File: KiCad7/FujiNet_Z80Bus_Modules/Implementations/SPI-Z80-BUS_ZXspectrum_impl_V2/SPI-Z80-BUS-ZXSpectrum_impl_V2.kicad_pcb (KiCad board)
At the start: 2 copper layers, 155 x 55 mm, 28 parts, among them J1 PinHeader_2.54mm, J2 LOCAL_D, J3 ESP_SPI_INT, J4 ESP_CONTROL, J5 Z80_CONTROL, J6 LOCAL_A-L, J7 LOCAL_A-H, U1 74HC00

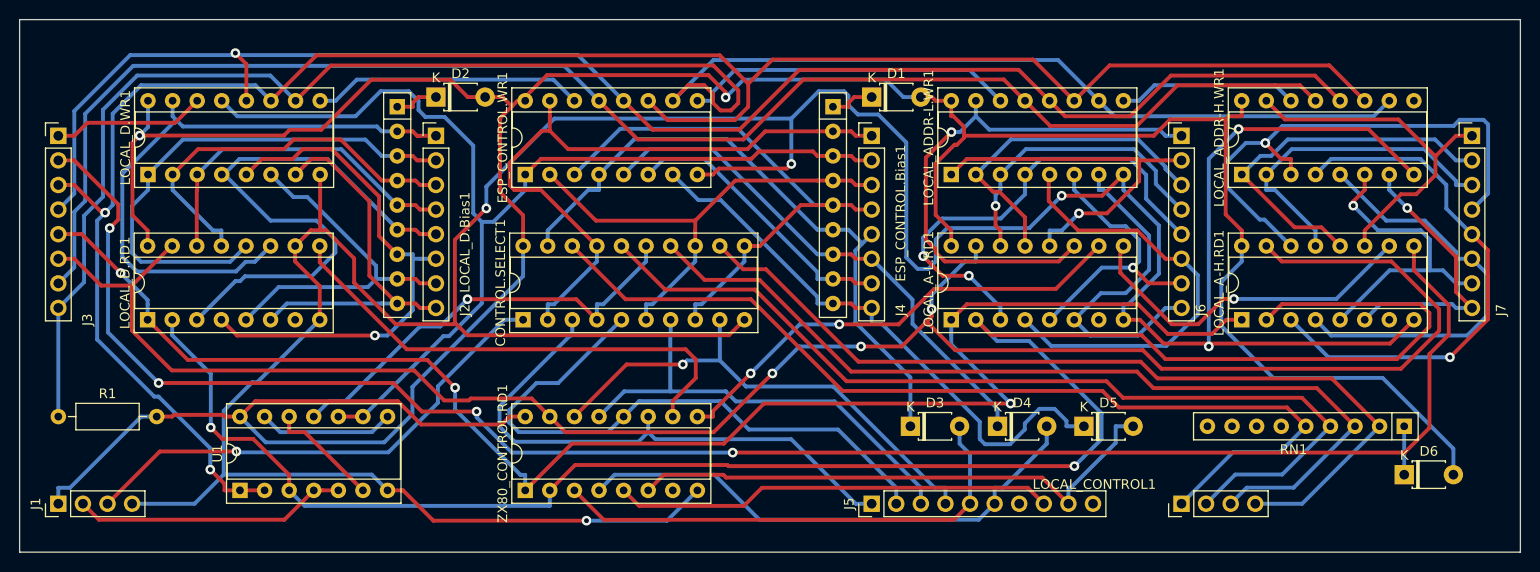
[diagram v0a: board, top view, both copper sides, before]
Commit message: KICAD - SPI_V2 board implementation
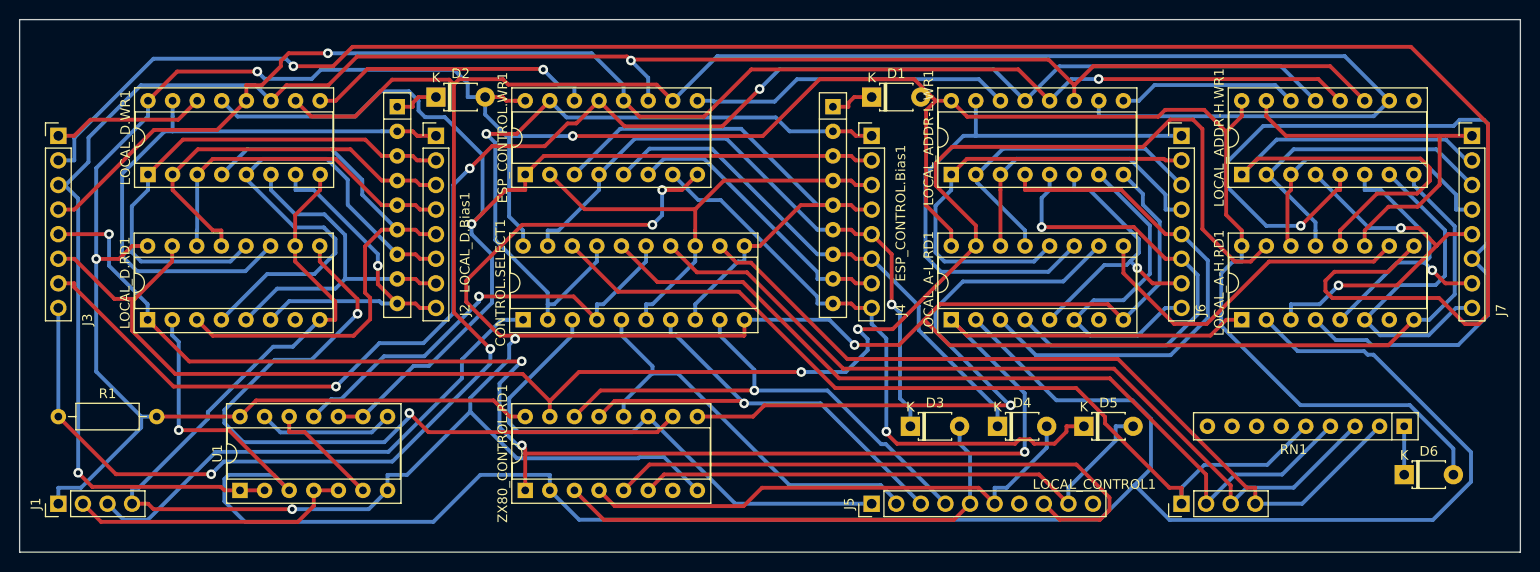
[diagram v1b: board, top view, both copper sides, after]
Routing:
- net /SPI-Z80-BUS/ESP_SPI_INT.MR: track 193.8 -> 246.1 mm, vias 0 -> 2
- net /SPI-Z80-BUS/LOCAL_A13: track 43.5 -> 89.3 mm, vias 0 -> 1
- net GND: track 366.6 -> 321.8 mm, vias 6 -> 5
- net /SPI-Z80-BUS/SPI-Z80-BUS_read/ESP_SPI_INT.SCK: track 201.8 -> 234.3 mm, vias 2 -> 1
- net Net-(LOCAL_D.RD1-Q7): track 51.6 -> 77.9 mm, vias 0 -> 2
- net /SPI-Z80-BUS/LOCAL_A11: track 55.2 -> 30.1 mm, vias 1 -> 0
- net /SPI-Z80-BUS/ESP_SPI_INT.MISO: track 185.9 -> 207.8 mm, vias 4 -> 1
- net /SPI-Z80-BUS/LOCAL_A9: track 39.4 -> 61.0 mm
- net /SPI-Z80-BUS/ESP_SPI_INT.CE: track 200.5 -> 180.1 mm, vias 3 -> 2
- net /SPI-Z80-BUS/Z80_CONTROL.WR: track 63.8 -> 43.6 mm
- net Net-(LOCAL_A-L.RD1-DS): track 49.1 -> 65.6 mm, vias 2 -> 1
- net /SPI-Z80-BUS/Z80_CONTROL.BUSACK: track 45.5 -> 61.9 mm
- net /SPI-Z80-BUS/LOCAL_A12: track 54.5 -> 38.9 mm, vias 1 -> 2
- net +5V: track 325.2 -> 312.7 mm, vias 2 -> 3
- net /SPI-Z80-BUS/ESP_SPI_INT.PL: track 160.2 -> 171.6 mm, vias 3 -> 4
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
